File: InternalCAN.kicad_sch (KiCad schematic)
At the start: 7 parts, among them J11 CAN_1, U4 ISO1044BD, U5 CDSOT23-T24CAN

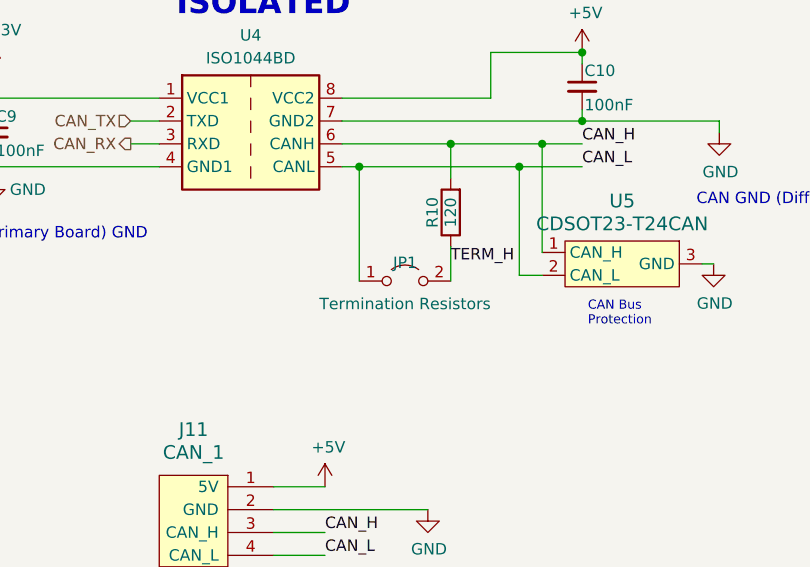
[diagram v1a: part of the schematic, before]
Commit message: Added power distribution ferrite bead
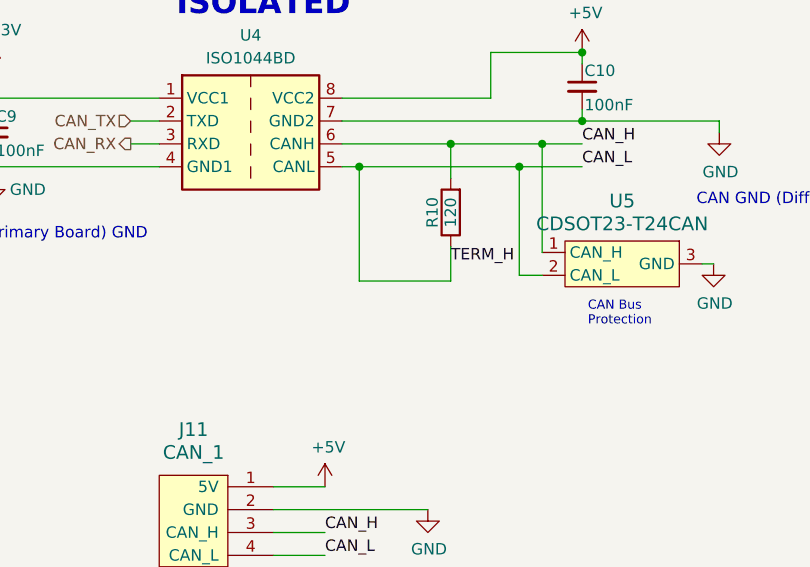
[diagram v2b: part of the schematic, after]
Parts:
- removed JP1: Termination Resistors, Connector_PinHeader_2.54mm:PinHeader_1x02_P2.54mm_Vertical, symbol Jumper:Jumper_2_Open
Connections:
- net TERM_H is gone; now on net CAN_L: R10.1
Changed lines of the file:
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@@
+    (stroke (width 0) (type default))
+  )
+  (wire (pts (xy 124.46 89.535) (xy 134.62 89.535))
     (stroke (width 0) (type default))
   )
@@
         )
       )
-    )
-  )
-  (symbol (lib_id "Jumper:Jumper_2_Open") (at 129.54 89.535 0) (unit 1)
-    (in_bom yes) (on_board yes) (dnp no)
-    (property "Reference" "JP1" (at 129.54 87.503 0)
-      (effects (font (size 1.27 1.27)))
-    )
-    (property "Value" "Termination Resistors" (at 129.54 92.075 0)
-      (effects (font (size 1.27 1.27)))
-    )
-    (property "Footprint" "Connector_PinHeader_2.54mm:PinHeader_1x02_P2.54mm_Vertical" (at 129.54 89.535 0)
-      (effects (font (size 1.27 1.27)) hide)
-    )
-    (property "Datasheet" "~" (at 129.54 89.535 0)
-      (effects (font (size 1.27 1.27)) hide)
-    )
-    (pin "1")
-    (pin "2")
-    (instances
-      (project "LeaderSOM"
-        (path "/192d0c36-944e-4927-949b-263b8c85a7ca/3c3cb7b2-3464-4424-b8df-3064a68eb04d"
-          (reference "JP1") (unit 1)
-        )
-      )
-      (project "Dashboard"
-        (path "/66218487-e316-4467-9eba-79d4626ab24e/00000000-0000-0000-0000-00005f547b94"
-          (reference "JP2") (unit 1)
-        )
-      )
-      (project "BPS-PeripheralSOM"
-        (path "/d5ebd247-5a7c-47c2-8aee-beabaef72d6d/1d0c269d-60cf-499b-bfd2-5087981d6678"
-          (reference "JP2") (unit 1)
-        )
-      )
